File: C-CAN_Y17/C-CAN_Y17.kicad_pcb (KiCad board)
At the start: 2 copper layers, 84.5 x 57.8 mm, 31 parts, among them J1 S1_Pull, J2 S2_Pull, J3 S3_Pull, J4 S4_Pull, J5 S5_Pull, P3 CAN_Terminate, P4 MX150_8, P5 MX150_16, SW1 SW_Push, U1 MCP2551-I/SN, U2 AP1117, U3 Cypress_5LP, Y1 Crystal

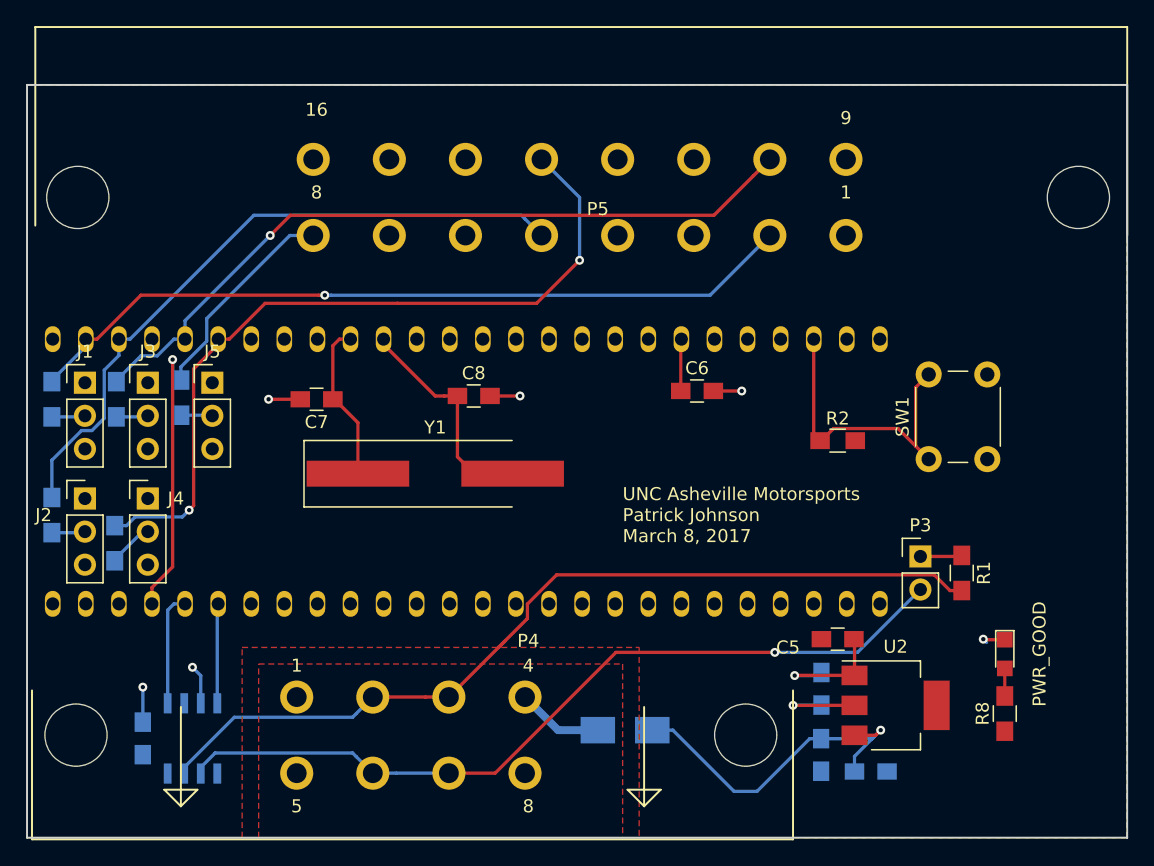
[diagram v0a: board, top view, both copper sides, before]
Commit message: ESF Fixes
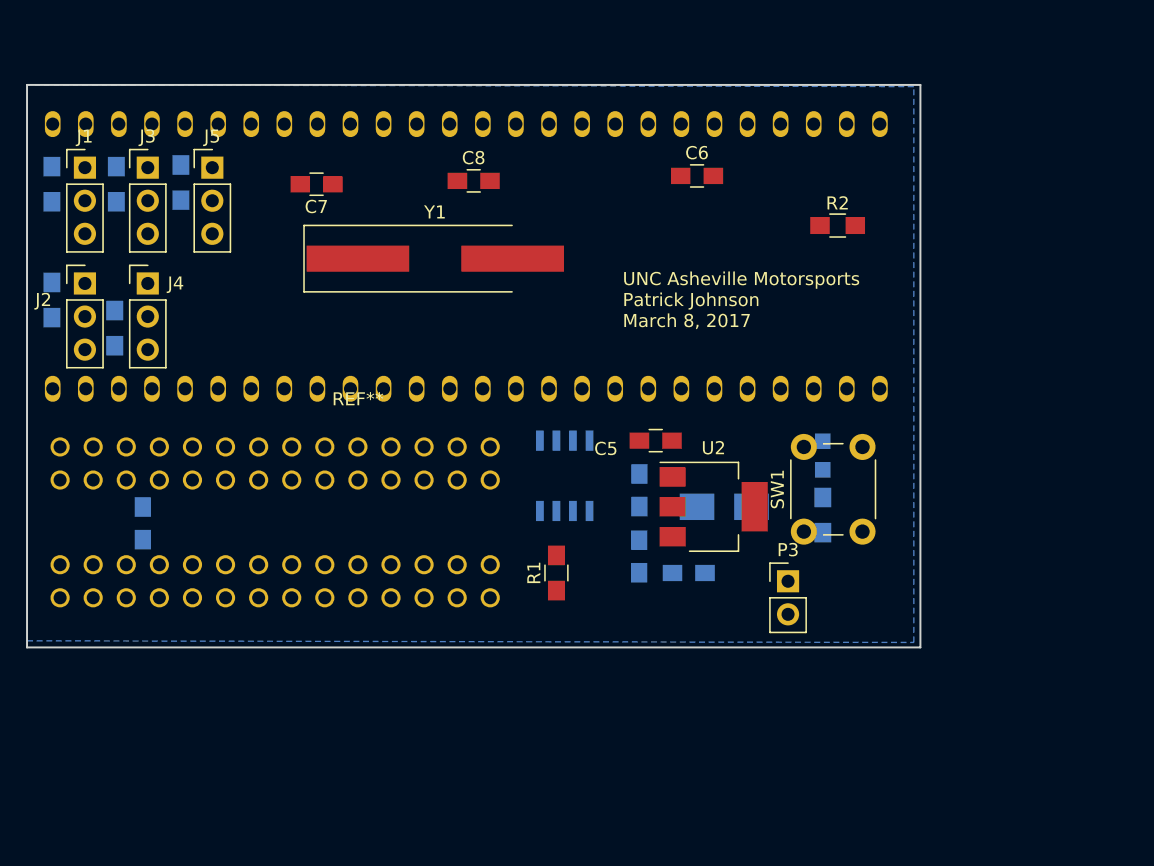
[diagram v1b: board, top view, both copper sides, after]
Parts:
- removed P4: MX150_8, UNCAMotorsports:MX150_8Pin
- removed P5: MX150_16, UNCAMotorsports:MX150_16pin
- added REF**: MX123_56, UNCAMotorsports:MX123_56, F.Cu at (99.1, 110.5)
- PWR_GOOD, R8: moved to B.Cu
- moved U1 35.0 mm to (137.8, 101.1)
- moved R1 31.1 mm to (137.2, 108.6), turned to 90 degrees
- moved C2 20.7 mm to (143.5, 107.3)
- moved C3 20.7 mm to (147.3, 108.6)
- moved C5 20.7 mm to (144.8, 98.4)
- moved PWR_GOOD 20.7 mm to (157.6, 99.6), turned to 90 degrees
- moved U2 20.7 mm to (149.2, 103.5)
- moved C4 20.7 mm to (143.5, 102.2)
- moved R8 20.7 mm to (157.6, 104.1), turned to 270 degrees
- moved F1 18.8 mm to (150.0, 103.5)
- moved C7 16.5 mm to (118.7, 78.7)
- moved J1 16.5 mm to (101.0, 77.5)
- moved J2 16.5 mm to (101.0, 86.4)
- moved J3 16.5 mm to (105.8, 77.5)
- moved J4 16.5 mm to (105.8, 86.4)
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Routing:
- net /CAN_H: track 68.2 -> 0.00 mm
- net /CAN_L: track 62.7 -> 0.00 mm, vias 1 -> 0
- net /S1: track 60.2 -> 0.00 mm, vias 1 -> 0
- net /S4: track 59.5 -> 0.00 mm, vias 2 -> 0
- net /S3: track 58.1 -> 0.00 mm, vias 1 -> 0
- net /S2: track 51.9 -> 0.00 mm
- net /H1: track 37.6 -> 0.00 mm, vias 1 -> 0
- net Net-(C2-Pad1): track 27.6 -> 0.00 mm, vias 1 -> 0
- net Net-(R2-Pad1): track 23.6 -> 0.00 mm
- net GND: track 18.5 -> 0.00 mm, vias 5 -> 0
- net Net-(C8-Pad1): track 17.2 -> 0.00 mm
- net +5V: track 12.6 -> 0.00 mm, vias 3 -> 0
- net Net-(C7-Pad1): track 12.3 -> 0.00 mm
- net /CAN_TX: track 8.68 -> 0.00 mm
- net /CAN_RX: track 7.66 -> 0.00 mm
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- removed copper zone on F.Cu, net +12V
- removed copper zone on F.Cu, net +5V
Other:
- board size 84.5 x 57.8 mm -> 68.6 x 43.2 mm
